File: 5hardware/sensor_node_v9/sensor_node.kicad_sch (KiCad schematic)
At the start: 23 parts, among them J1 Conn_01x04_Pin, J3 Conn_01x04_Pin, Q1 BC818, Q2 Si2371EDS, Q3 AO3400A, U12 APDS-9960, U13 SHT31-DIS, U17 BH1750FVI-TR, U7 XC6206PxxxMR, U8 TPL5110

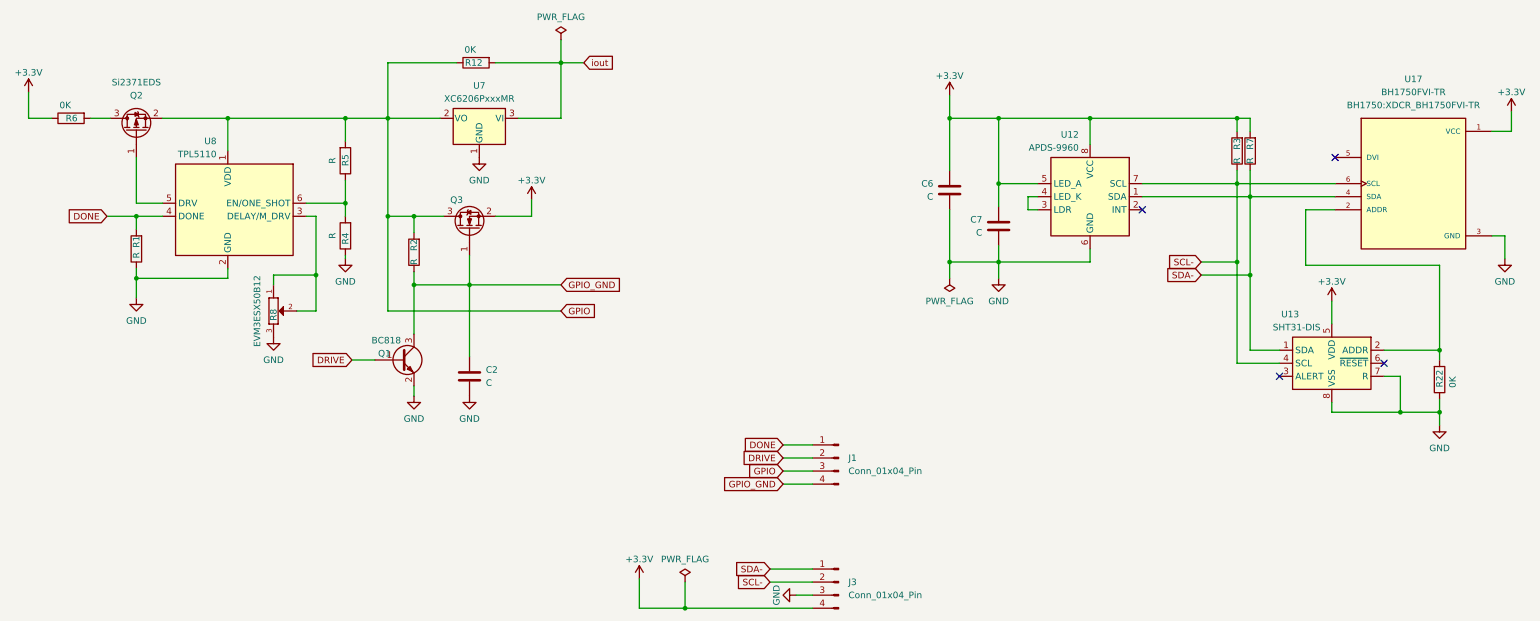
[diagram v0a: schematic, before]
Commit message: update PCB.
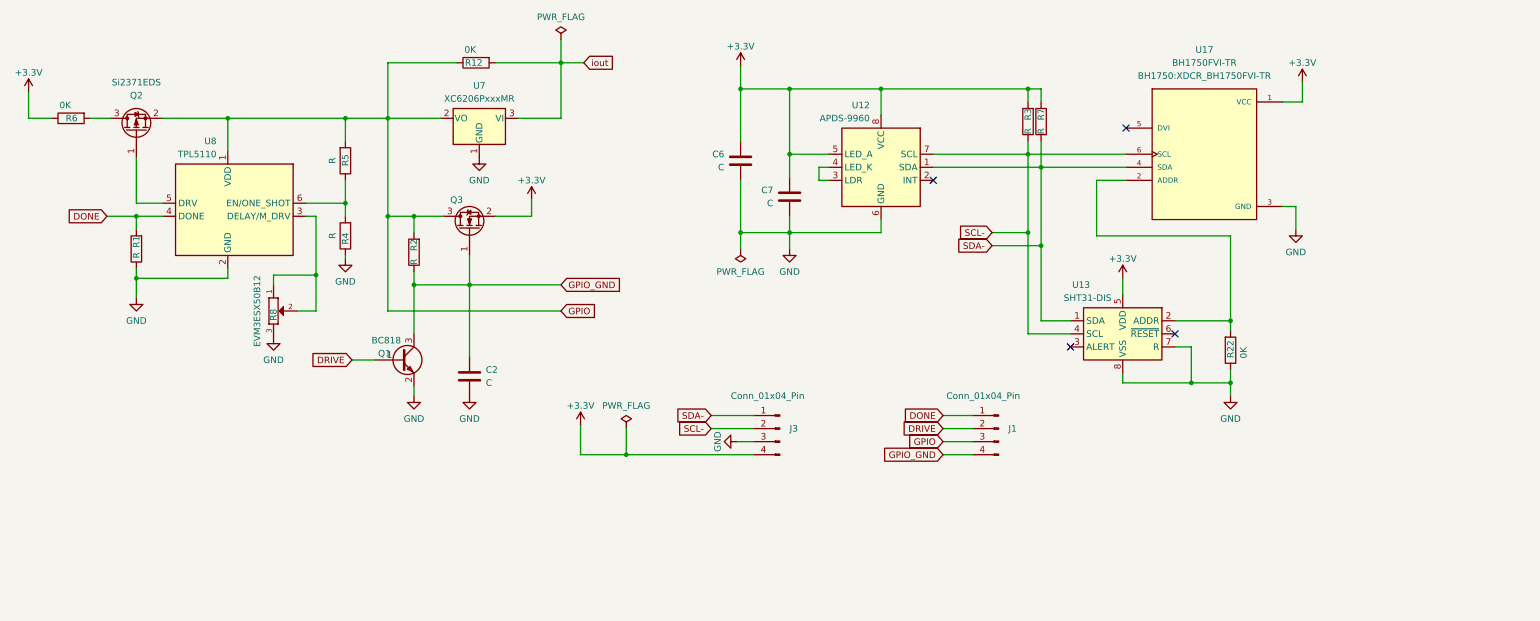
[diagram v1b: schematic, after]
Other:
- moved on the sheet: C6, C7, J1, J3, R22, R3, R7, U12, U13, U17
